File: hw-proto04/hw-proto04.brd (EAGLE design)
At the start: 54.3 x 62.2 mm, 30 parts, among them IC2 UCC27523DR, IC3 MCP2562T, IC4 STM32F042C6T7, IC5 TLV74333PDBVR, J1 10, J2 10, Q1 SQJ147ELP-T1_GE3, Q2 SQJ147ELP-T1_GE3

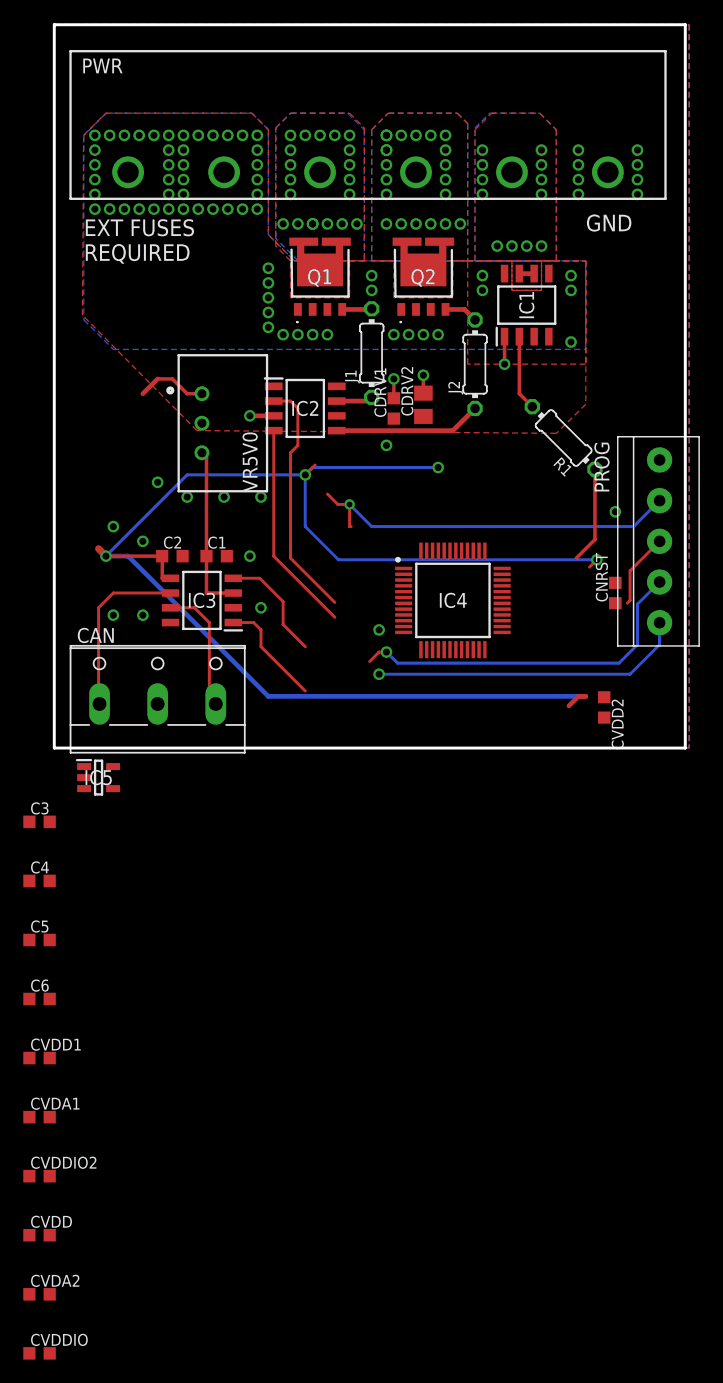
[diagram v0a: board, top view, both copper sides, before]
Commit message: layout, routing and schematic refinement
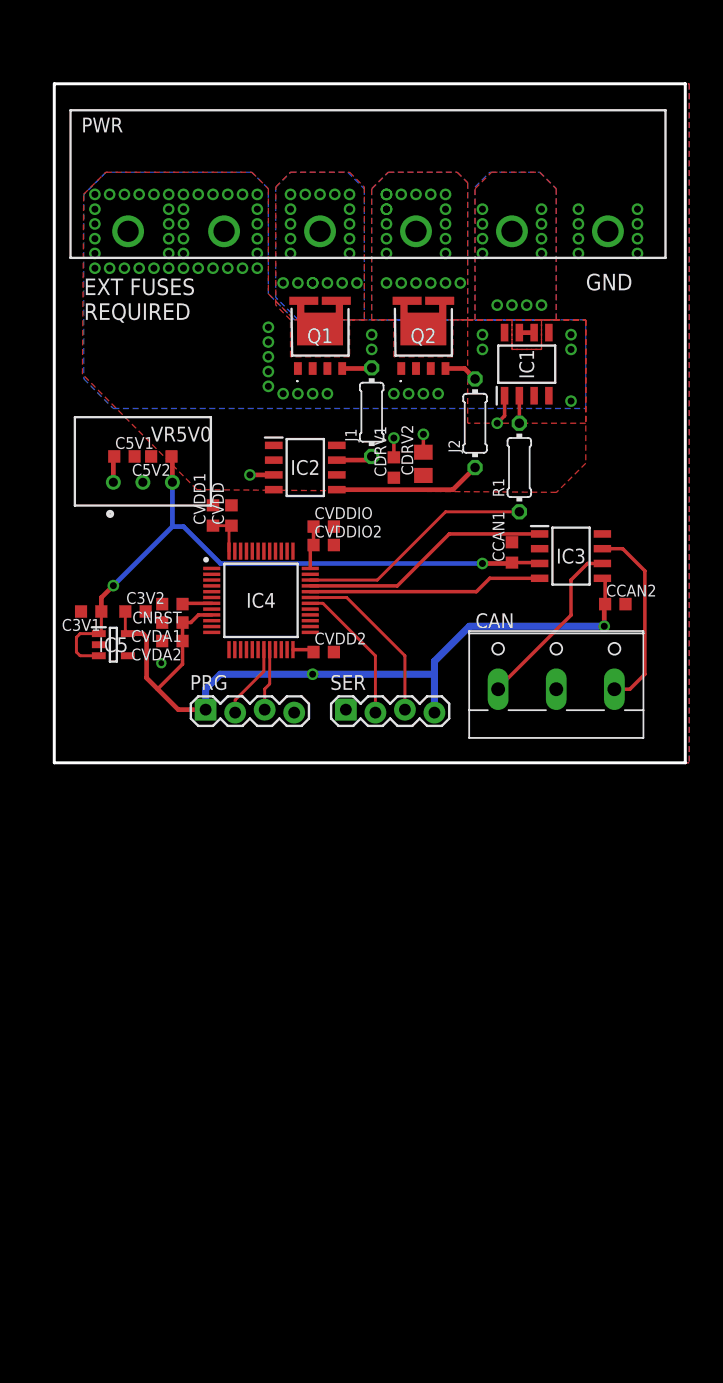
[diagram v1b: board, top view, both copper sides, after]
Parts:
- removed C1, C2: 100n, rcl:C0603K
- removed C3, C4, C5, C6: 1u, rcl:C0603K
- removed PROG: 1X5, adafruit:1X05-3.5MM
- added C3V1, C3V2, C5V1, C5V2: 1u, rcl:C0603K
- added CCAN1, CCAN2: 100n, rcl:C0603K
- added PRG, SER: (no value), SparkFun-Connectors:1X04_LOCK
- moved CVDDIO 75.2 mm to (24.4, 20.3)
- moved CVDD 64.1 mm to (16.5, 21.3), turned to 90 degrees
- moved CVDDIO2 59.5 mm to (24.4, 18.7)
- moved CVDA2 57.3 mm to (11.4, 10.5), turned to 180 degrees
- moved CVDD1 49.0 mm to (14.9, 21.3), turned to 90 degrees
- moved CVDA1 44.1 mm to (11.4, 12.1), turned to 180 degrees
- moved CNRST 38.1 mm to (11.4, 13.7), turned to 180 degrees
- moved CAN 34.3 mm to (44.5, 7.62)
- moved IC3 32.0 mm to (45.7, 17.8), turned to 0 degrees
- moved CVDD2 24.6 mm to (24.4, 9.53), turned to 0 degrees
- moved IC4 16.5 mm to (19.1, 14.0)
- moved IC5 11.5 mm to (6.35, 10.2)
- moved VR5V0 7.18 mm to (8.89, 24.1), turned to 0 degrees
- moved CDRV1 5.08 mm to (30.5, 25.4)
- moved IC2 5.08 mm to (22.9, 25.4)
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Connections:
- removed net EN: PROG.3
- removed net GPIO0: PROG.4
- removed net RX: IC4.31
- removed net RXD0: PROG.2
- removed net TX: IC4.30
- removed net TXD0: PROG.1
- new net RX1: IC4.31, SER.3
- new net SWCLK: IC4.20, PRG.3
- new net SWDIO: IC4.19, PRG.2
- new net TX1: IC4.30, SER.2
- net +12V: now also C5V1.1; no longer C5.1
- net +3V3: now also C3V2.1, CCAN2.1, PRG.1, SER.4; no longer C2.1, C4.1
- net +5V: now also C3V1.1, C5V2.1, CCAN1.1; no longer C1.1, C3.1, C6.1
- net CTL1: now also IC4.39
- net CTL2: now also IC4.40
- net CTL3: now also IC4.34
- net GND: now also C3V1.2, C3V2.2, C5V1.2, C5V2.2, CCAN1.2, CCAN2.2, PRG.4, SER.1; no longer C1.2, C2.2, C3.2, C4.2, C5.2, C6.2, PROG.5
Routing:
- net +3V3: track 121.7 -> 79.0 mm, vias 4 -> 2
- net +5V: track 14.5 -> 56.3 mm, vias 0 -> 2
- net GPIO0: track 32.7 -> 0.00 mm, vias 1 -> 0
- net RXD0: track 30.6 -> 0.00 mm, vias 1 -> 0
- net TXD0: track 27.3 -> 0.00 mm, vias 1 -> 0
- net CTL1: track 20.9 -> 0.00 mm
- net CTL2: track 18.2 -> 0.00 mm
- net RX1: track 0.00 -> 14.9 mm
- net TX1: track 0.00 -> 12.4 mm
- net CTL3: track 8.31 -> 20.4 mm
- net CAN_TX: track 9.48 -> 21.6 mm
- net CAN_RX: track 9.80 -> 20.2 mm
- net EN: track 6.47 -> 0.00 mm
- net SWDIO: track 0.00 -> 6.44 mm
- net N$1: track 11.1 -> 16.5 mm
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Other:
- board size 54.3 x 62.2 mm -> 54.3 x 58.4 mm
